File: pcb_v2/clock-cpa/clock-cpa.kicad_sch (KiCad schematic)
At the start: 31 parts, among them J1 EXT IN, J2 control panel, J3 control panel, J4 CLK OUT, SW1 1HZ, SW2 1KHZ, SW3 XTAL1, SW4 XTAL2, SW5 EXT, SW6 BREAK, SW7 CLOCK_RESET, SW8 HALF-STEP, SW9 STEP

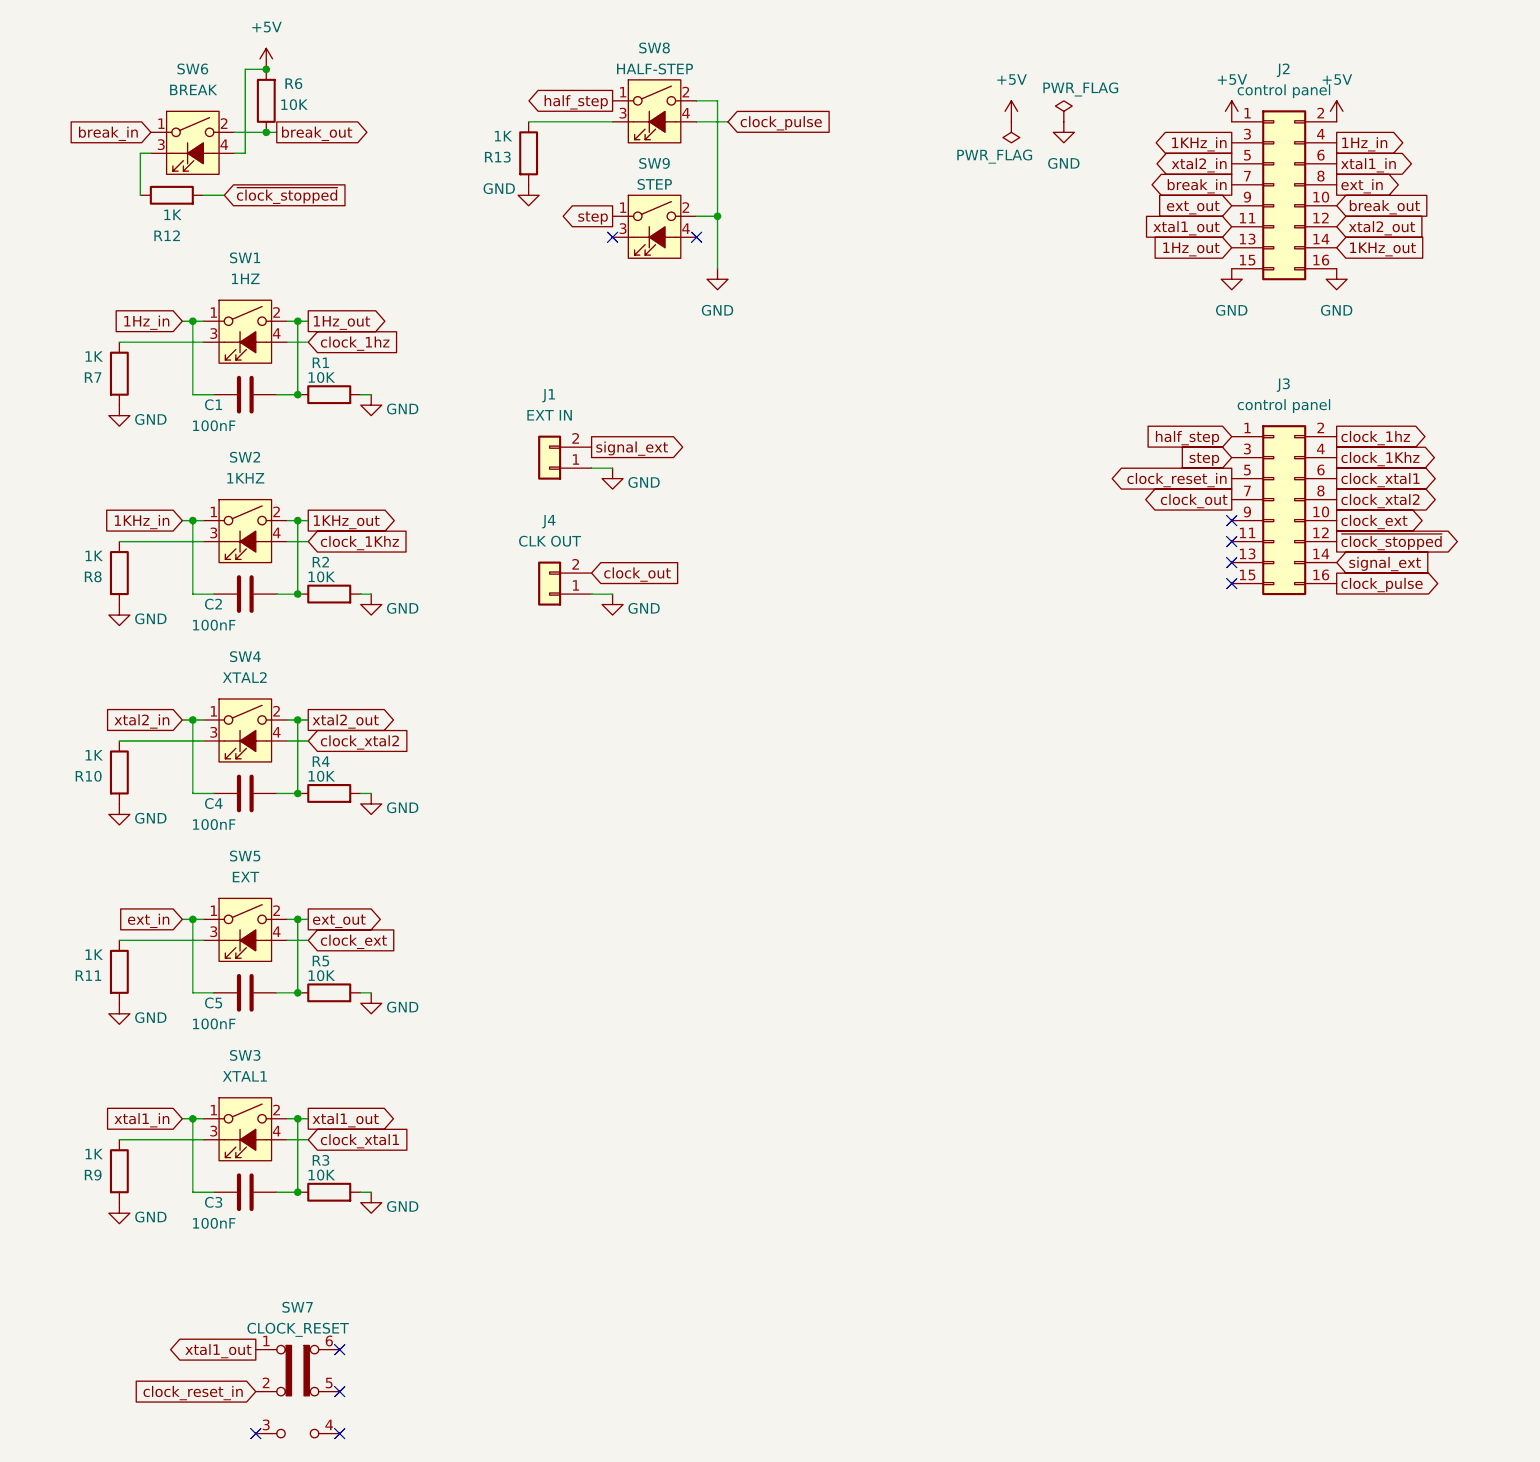
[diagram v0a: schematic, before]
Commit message: layout de pcb do clock
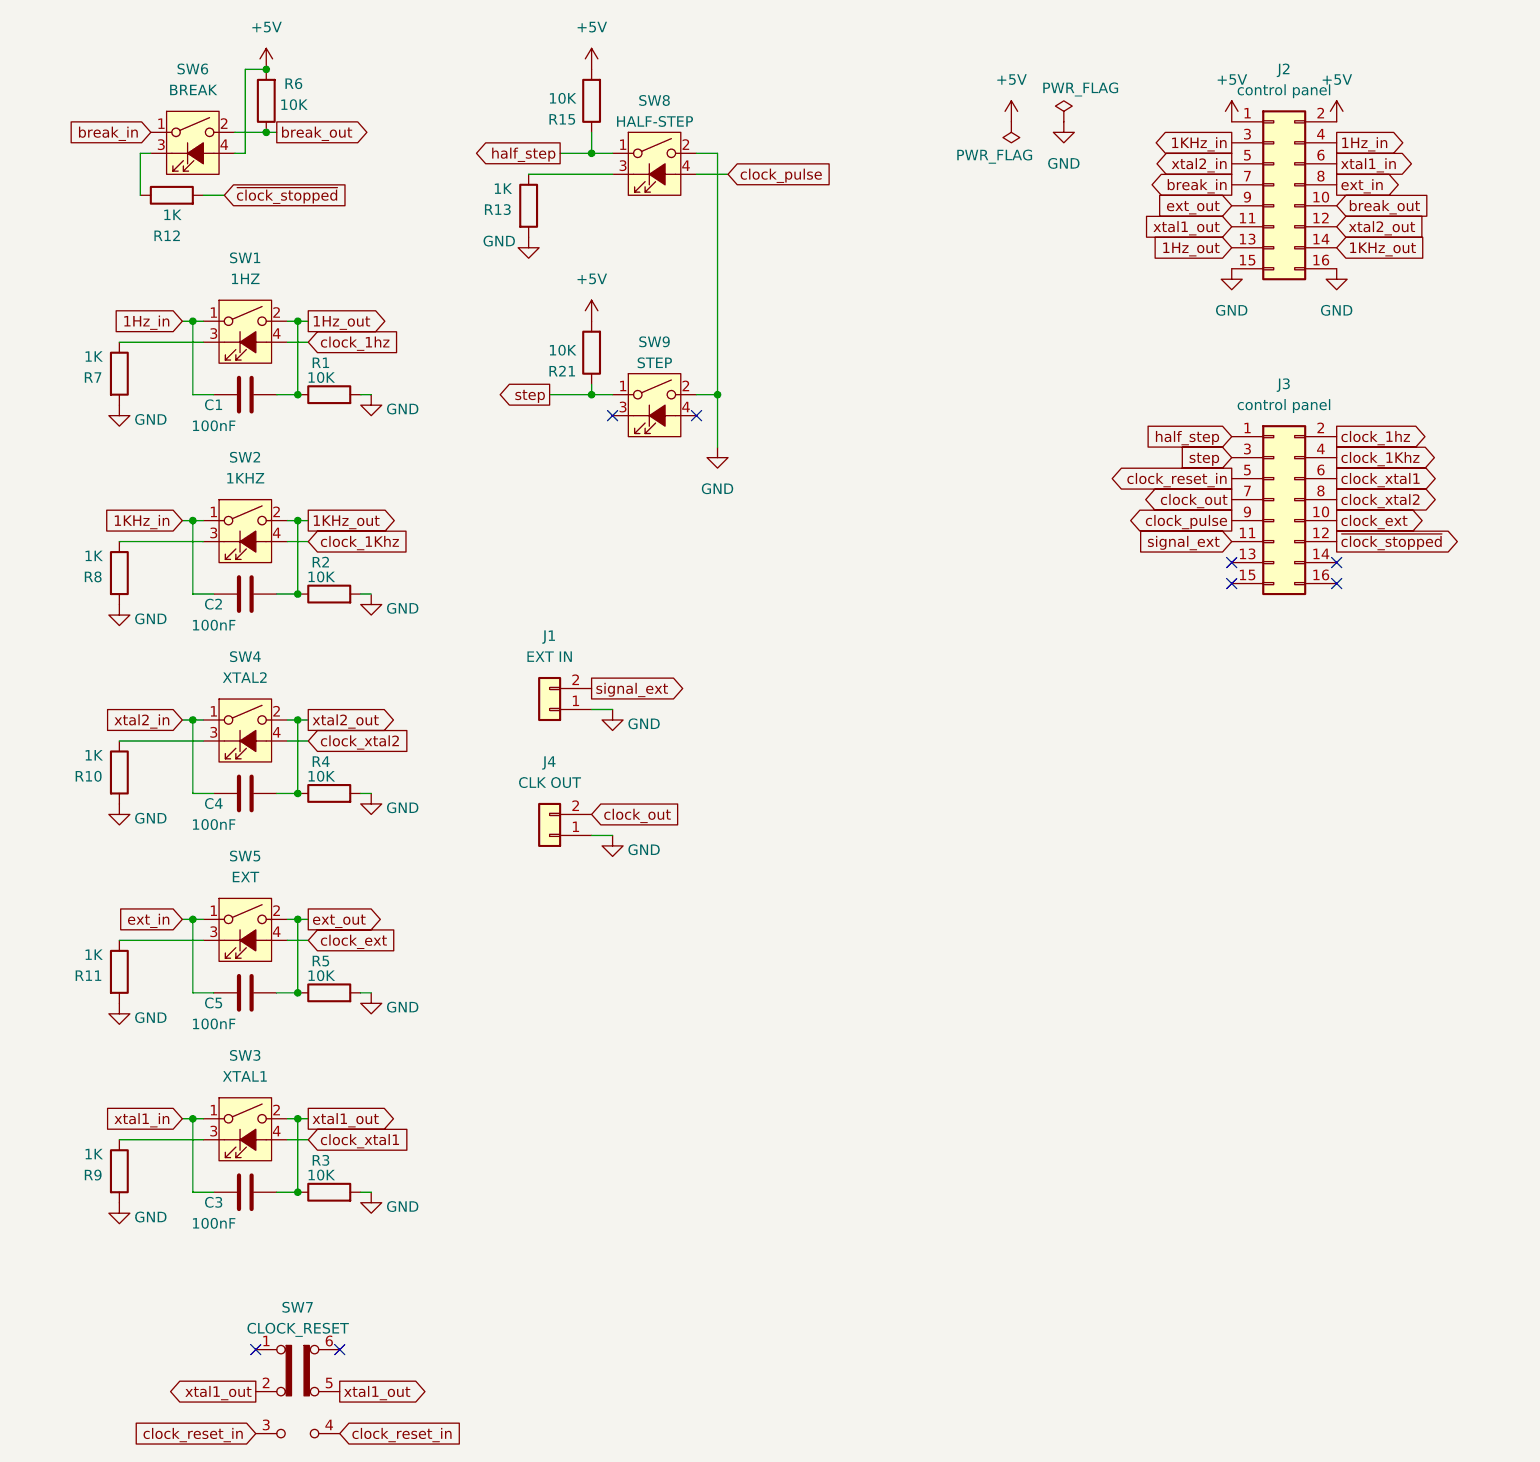
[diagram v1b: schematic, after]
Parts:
- added R15, R21: 10K, Resistor_THT:R_Axial_DIN0207_L6.3mm_D2.5mm_P7.62mm_Horizontal, symbol Device:R
- J1, J4: footprint Connector_Molex:Molex_KK-254_AE-6410-02A_1x02_P2.54mm_Vertical -> Connector_JST:JST_XH_B2B-XH-A_1x02_P2.50mm_Vertical
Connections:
- net +5V: now also R15.2, R21.2
- net clock_pulse: now also J3.9 (Pin_9); no longer J3.16 (Pin_16)
- net clock_reset_in: now also SW7.3 (C), SW7.4 (A); no longer SW7.2 (B)
- net half_step: now also R15.1
- net signal_ext: now also J3.11 (Pin_11); no longer J3.14 (Pin_14)
- net step: now also R21.1
- net xtal1_out: now also SW7.2 (B), SW7.5 (B); no longer SW7.1 (A)
- no-connect marks 10 -> 8
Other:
- moved on the sheet: J1, J4, R13, SW8, SW9

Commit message: continuando implementação do clock
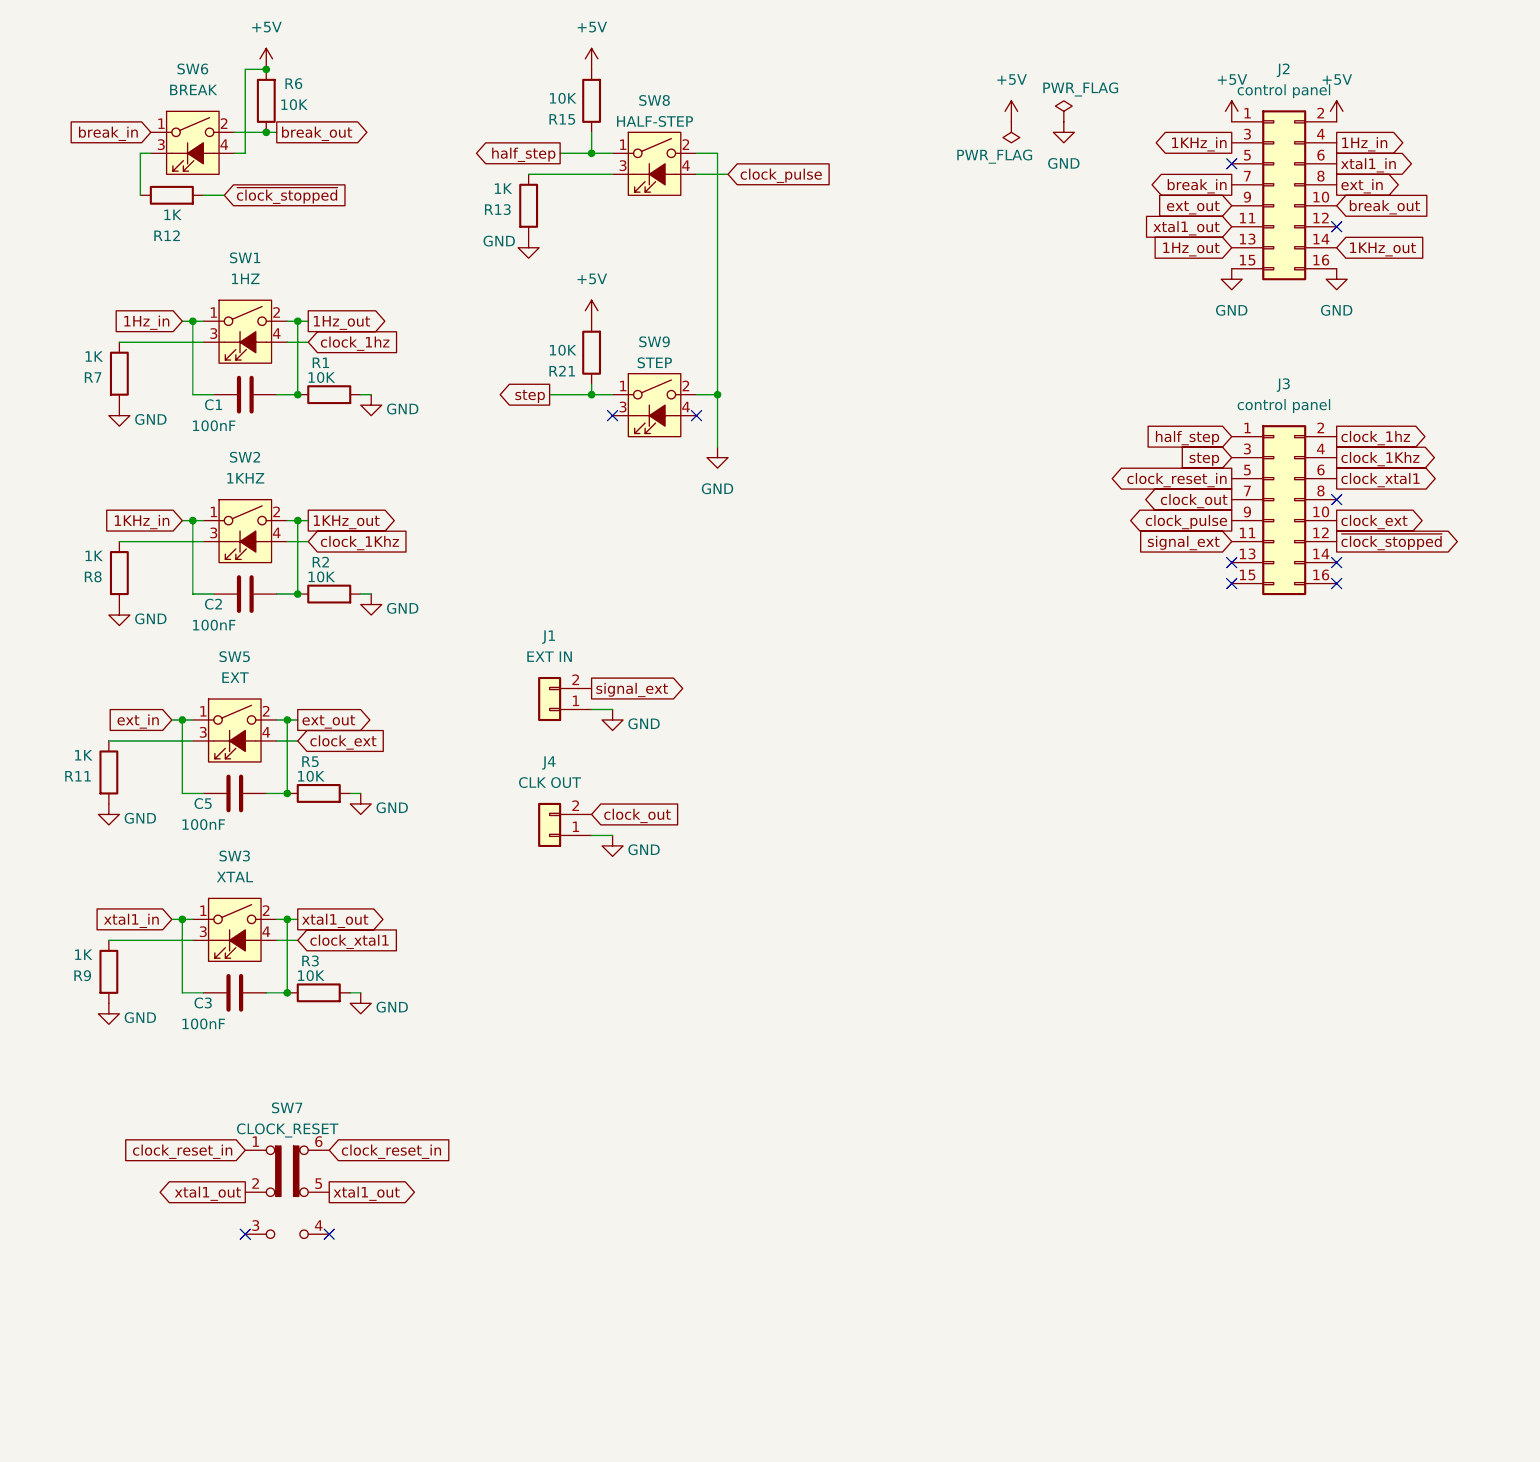
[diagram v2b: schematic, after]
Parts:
- removed C4: 100nF, Capacitor_THT:C_Disc_D4.7mm_W2.5mm_P5.00mm, symbol Device:C
- removed R10: 1K, Resistor_THT:R_Axial_DIN0207_L6.3mm_D2.5mm_P7.62mm_Horizontal, symbol Device:R
- removed R4: 10K, Resistor_THT:R_Axial_DIN0207_L6.3mm_D2.5mm_P7.62mm_Horizontal, symbol Device:R
- removed SW4: XTAL2, clock-buttons:TS5 LED Momentary Click Tact Switch, symbol Switch:SW_SPST_LED
- SW3: value XTAL1 -> XTAL
- SW7: footprint Button_Switch_THT:SW_CK_JS202011CQN_DPDT_Straight -> clock-buttons:Slide Switch DPDT
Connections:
- net clock_reset_in: now also SW7.1 (A), SW7.6 (C); no longer SW7.3 (C), SW7.4 (A)
- net clock_xtal2: no longer names the net of J3.8 (Pin_8)
- net xtal2_in: no longer names the net of J2.5 (Pin_5)
- net xtal2_out: no longer names the net of J2.12 (Pin_12)
- no-connect marks 8 -> 11
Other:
- moved on the sheet: C3, C5, R11, R3, R5, R9, SW3, SW5, SW7

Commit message: correções no esquemático e pcb
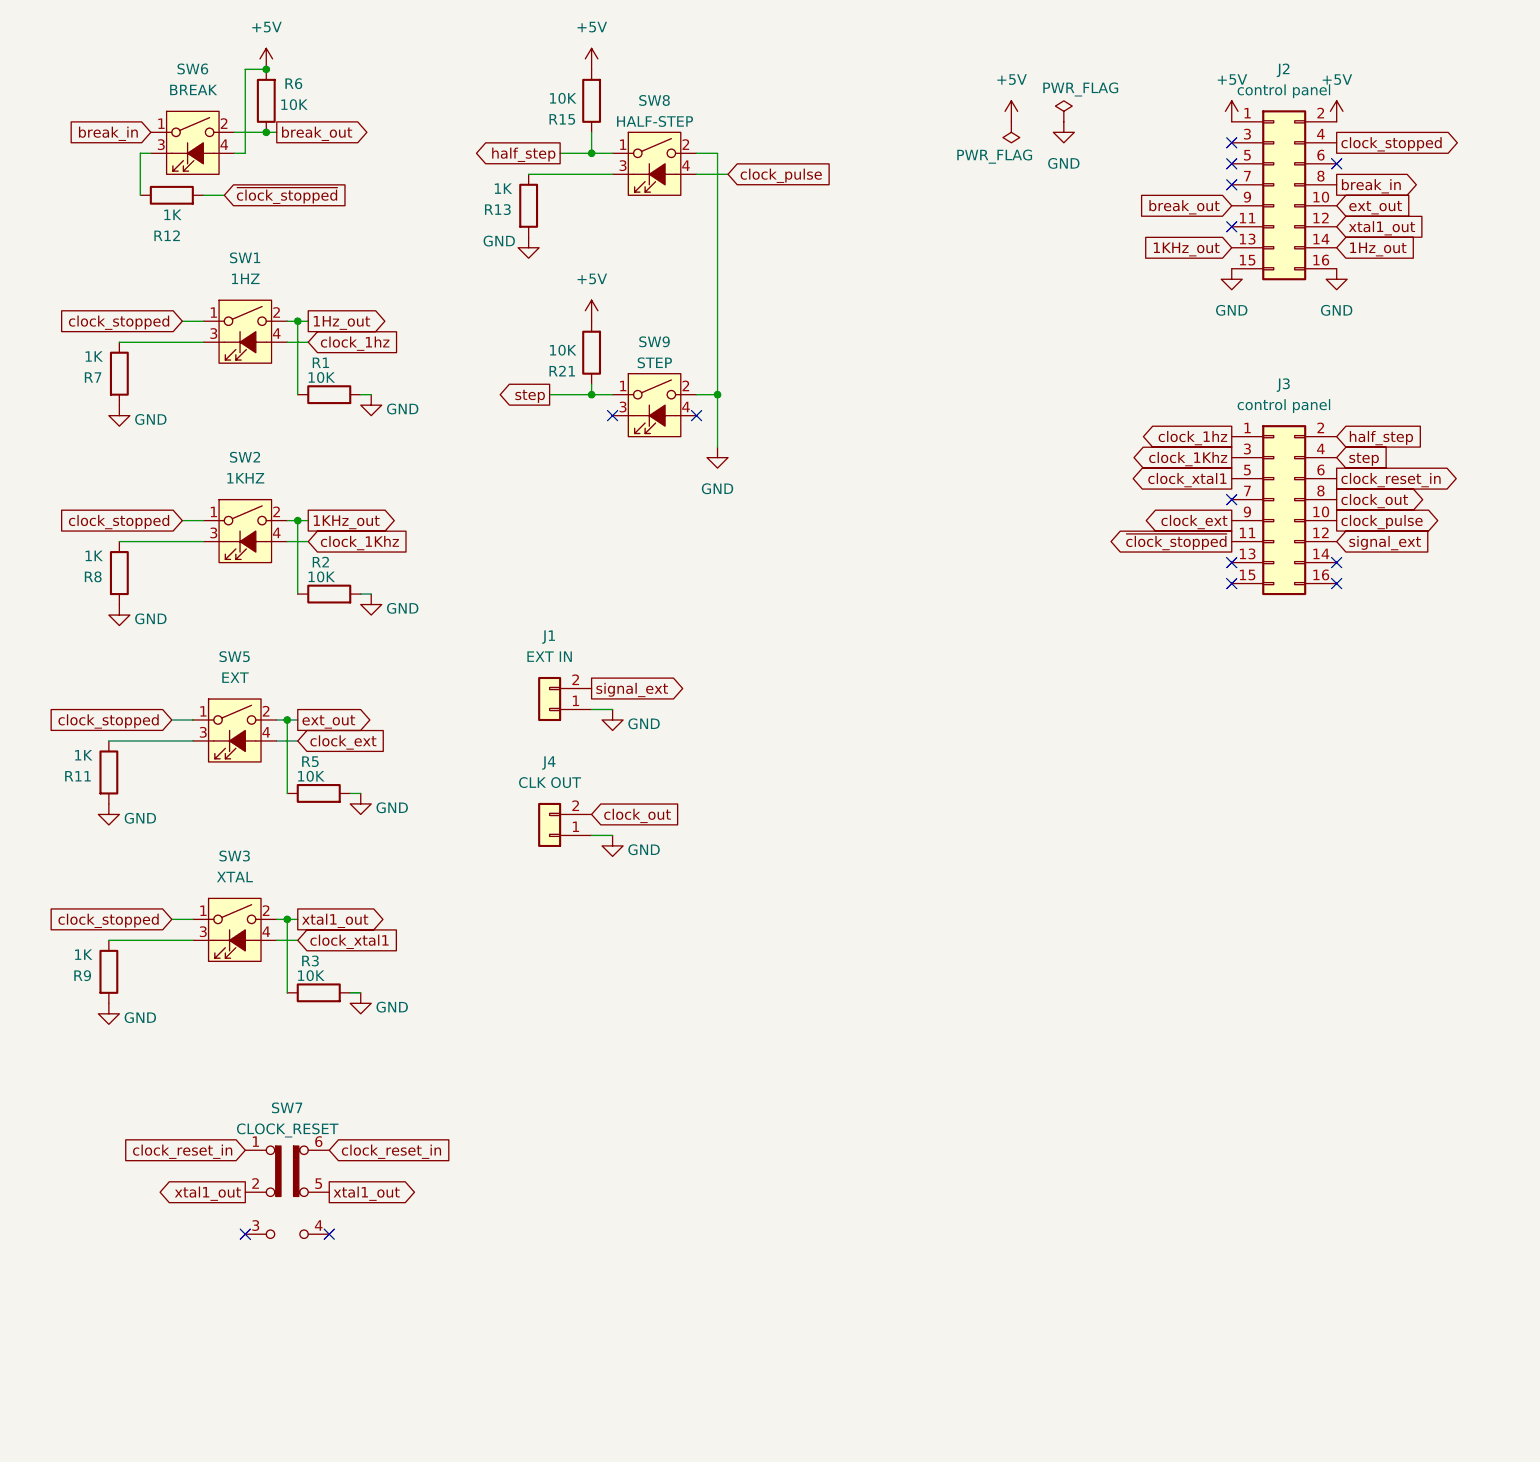
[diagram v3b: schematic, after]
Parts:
- removed C1, C2, C3, C5: 100nF, Capacitor_THT:C_Disc_D4.7mm_W2.5mm_P5.00mm, symbol Device:C
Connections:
- net 1Hz_out: now also J2.14 (Pin_14); no longer J2.13 (Pin_13)
- net 1KHz_out: now also J2.13 (Pin_13); no longer J2.14 (Pin_14)
- net break_in: now also J2.8 (Pin_8); no longer J2.7 (Pin_7)
- net break_out: now also J2.9 (Pin_9); no longer J2.10 (Pin_10)
- net clock_1Khz: now also J3.3 (Pin_3); no longer J3.4 (Pin_4)
- net clock_1hz: now also J3.1 (Pin_1); no longer J3.2 (Pin_2)
- net clock_ext: now also J3.9 (Pin_9); no longer J3.10 (Pin_10)
- net clock_out: now also J3.8 (Pin_8); no longer J3.7 (Pin_7)
- net clock_pulse: now also J3.10 (Pin_10); no longer J3.9 (Pin_9)
- net clock_reset_in: now also J3.6 (Pin_6); no longer J3.5 (Pin_5)
- net clock_xtal1: now also J3.5 (Pin_5); no longer J3.6 (Pin_6)
- net ext_out: now also J2.10 (Pin_10); no longer J2.9 (Pin_9)
- net half_step: now also J3.2 (Pin_2); no longer J3.1 (Pin_1)
- net signal_ext: now also J3.12 (Pin_12); no longer J3.11 (Pin_11)
- net step: now also J3.4 (Pin_4); no longer J3.3 (Pin_3)
- net xtal1_out: now also J2.12 (Pin_12); no longer J2.11 (Pin_11)
- net ~{clock_stopped}: now also J3.11 (Pin_11); no longer J3.12 (Pin_12)
- net 1Hz_in renamed clock_stopped
- net clock_stopped: now also SW2.1, SW3.1, SW5.1
- net 1KHz_in: no longer names the net of J2.3 (Pin_3)
- net 1KHz_in: no longer SW2.1
- removed net ext_in: J2.8 (Pin_8), SW5.1
- net xtal1_in: no longer names the net of J2.6 (Pin_6)
- net xtal1_in: no longer SW3.1
- no-connect marks 11 -> 14
